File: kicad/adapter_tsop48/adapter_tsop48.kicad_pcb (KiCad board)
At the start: 2 copper layers, 48 x 33 mm, 3 parts, among them J1 Conn_02x12_Odd_Even_1, J2 Conn_02x12_Odd_Even_2, P1 TSOP-48_adapter

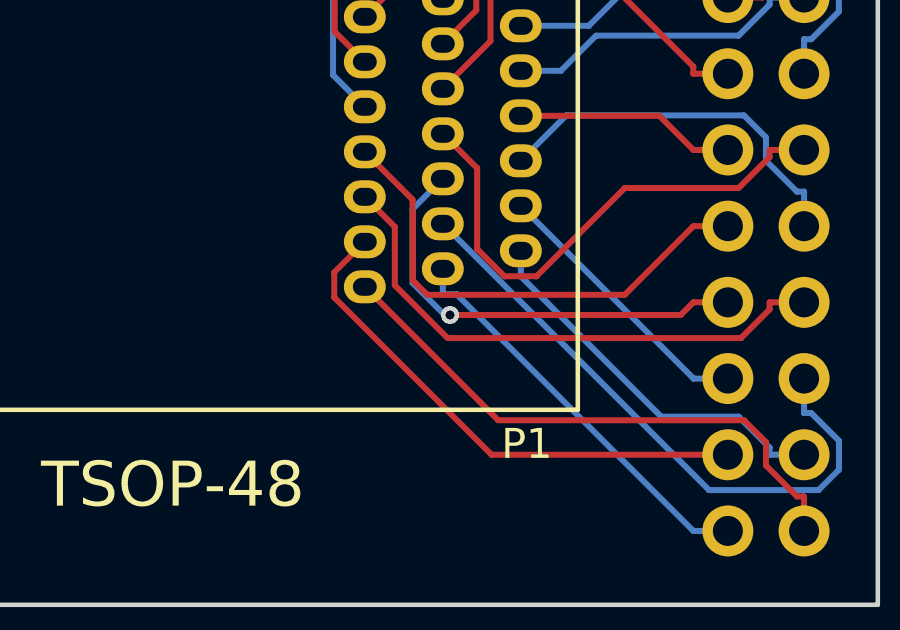
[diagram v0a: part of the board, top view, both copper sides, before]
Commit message: upgrade project files to kicad version 6.0.11
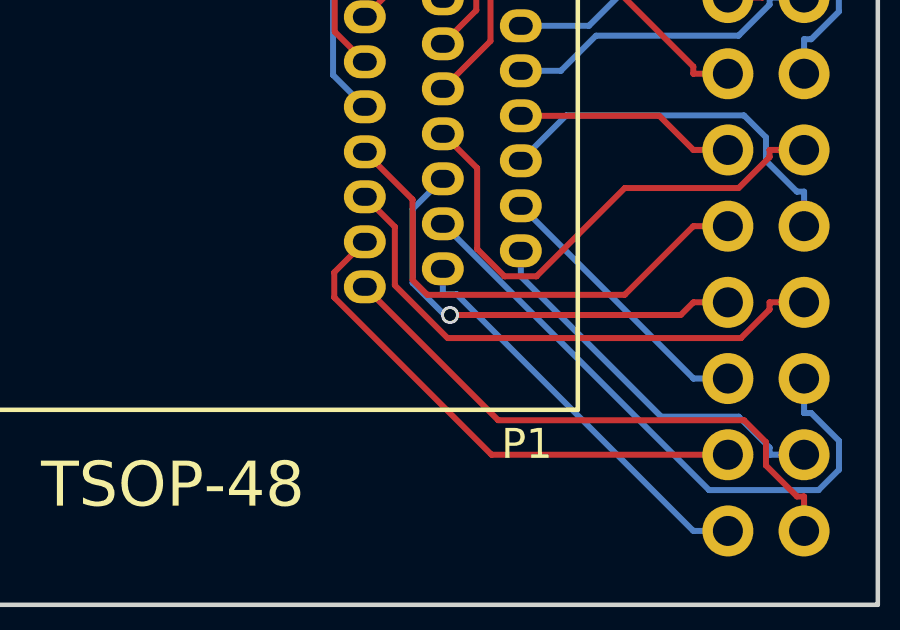
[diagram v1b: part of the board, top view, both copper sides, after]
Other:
- net class Default removed
